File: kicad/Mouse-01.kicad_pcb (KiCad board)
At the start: 2 copper layers, 58 x 62 mm, 117 parts, among them P1 MT-ENC, P10 USB_A, P11 BAT1, P12 BAT2, P2 MT-ENC, P3 Battery_A, P4 Battery_B, P5 SWD, P6 UART, P7 USB_A, P8 BAT1, P9 BAT2, Q1 IRLML6402, Q2 IRFML8244, Q3 IRFML8244, Q4 BSS138, SW1 RESET, SW2 Power, SW3 BUTTON, U1 STM32F405RGTx, U10 MCP73831, U11 MCP73831, U12 MCP73831, U2 DRV8835, U3 DRV8835, U4 LXDC55FAAA-203, U5 REF1933, U6 LT1963ES8, U7 AD8604, U8 MPU6500, U9 MCP73831

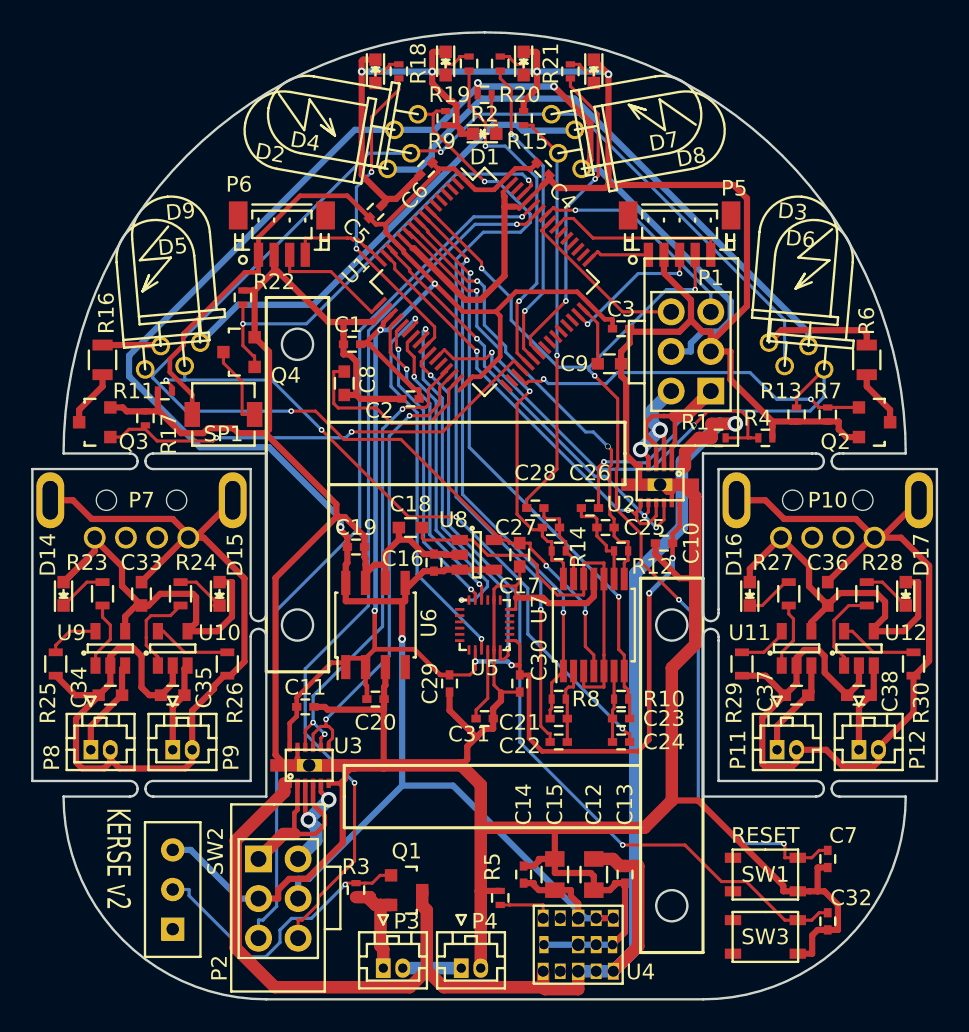
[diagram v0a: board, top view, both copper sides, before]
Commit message: viaを量産
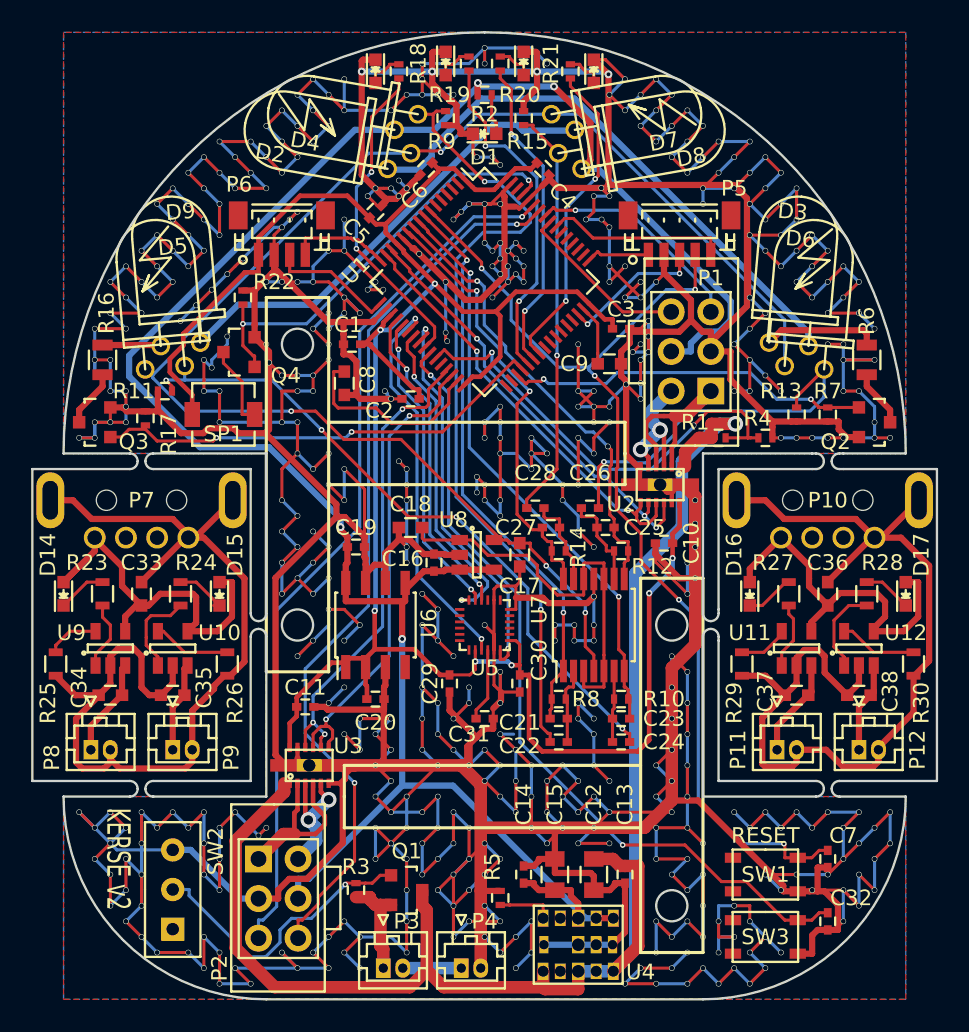
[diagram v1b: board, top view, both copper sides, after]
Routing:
- net GND: track 384.8 -> 1229.8 mm, vias 4 -> 531
- added copper zone on B.Cu, net GND
- added copper zone on F.Cu, net GND
